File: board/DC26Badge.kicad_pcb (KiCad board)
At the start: 2 copper layers, 6 parts, among them U1 HT16K33-28

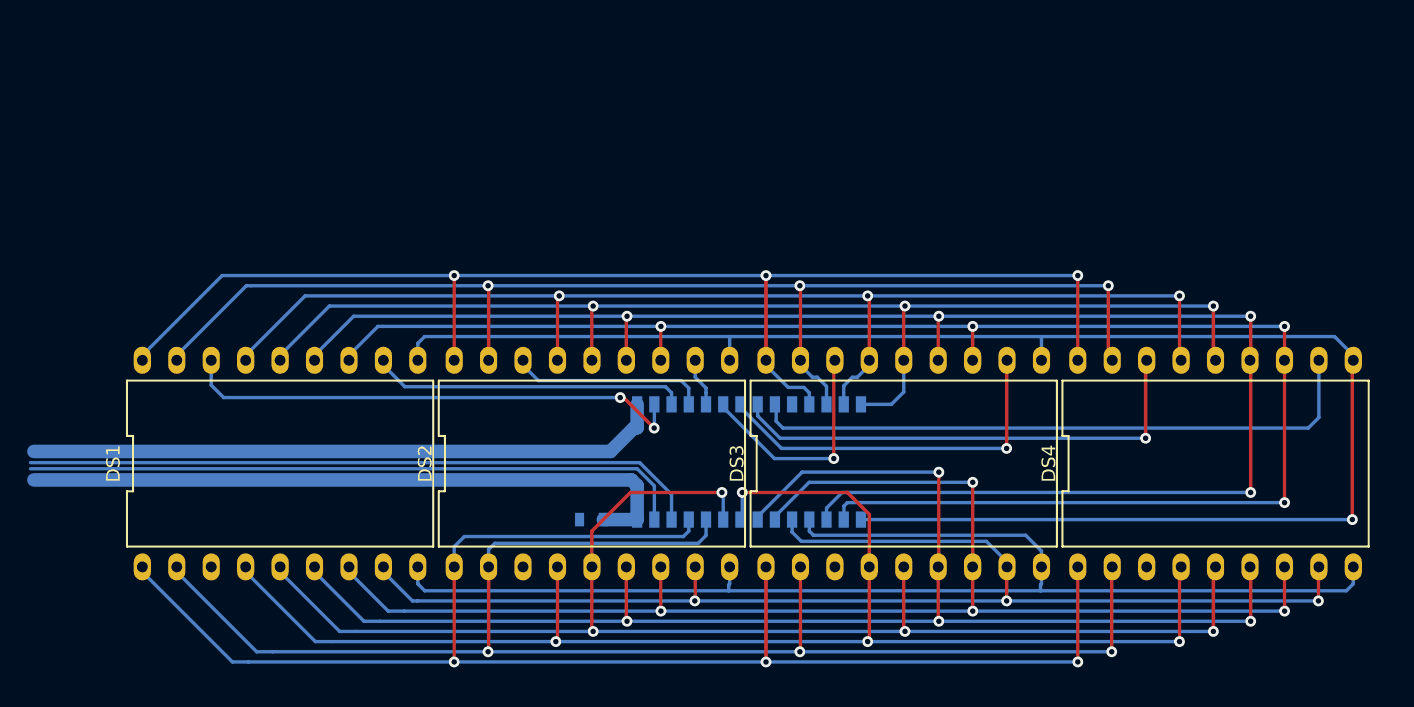
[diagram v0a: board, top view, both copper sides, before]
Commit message: First pass of prototype PCB layout.
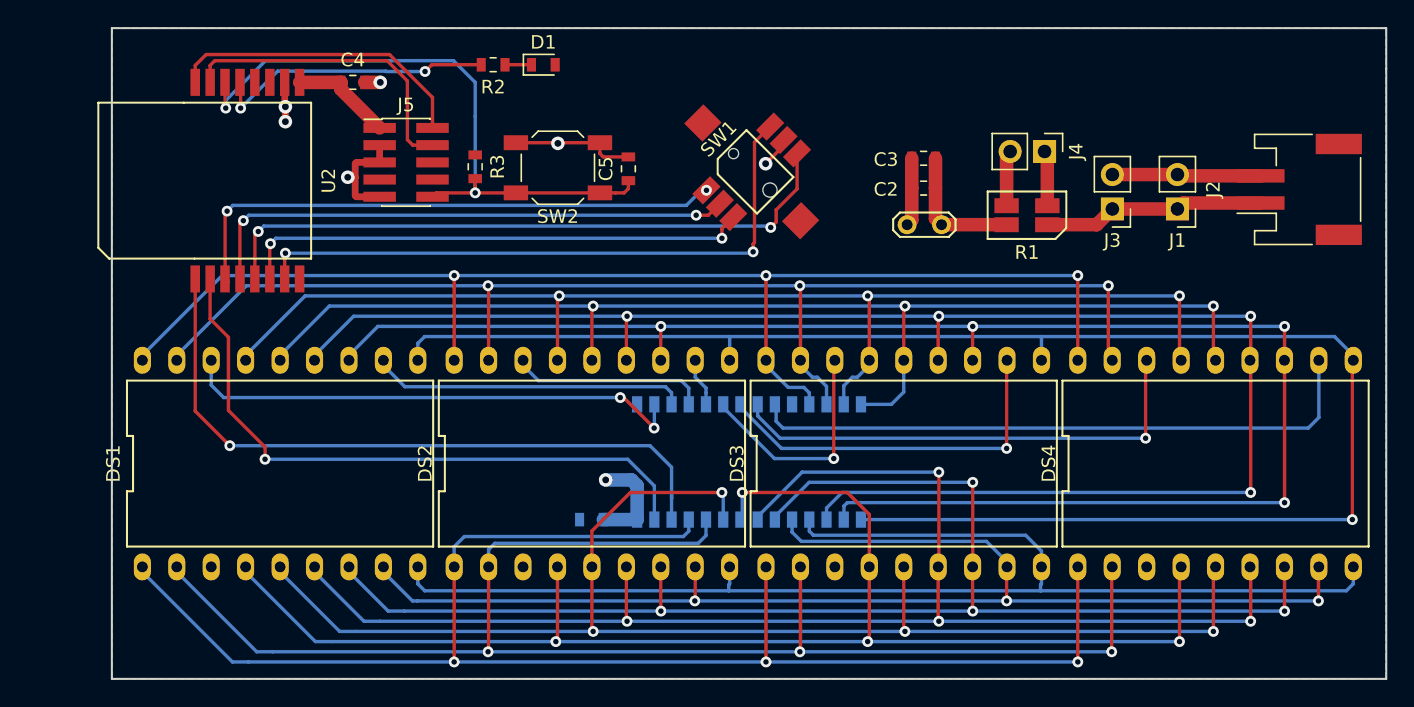
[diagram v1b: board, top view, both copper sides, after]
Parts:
- added C2: 4.7u, Capacitor_SMD:C_0603_1608Metric, F.Cu at (154.9, 33.8)
- added C3: 0.1u, Capacitor_SMD:C_0603_1608Metric, F.Cu at (154.9, 31.6)
- added C4: 0.1u, Capacitor_SMD:C_0603_1608Metric, F.Cu at (112.8, 26.0)
- added C5: 0.1u, Capacitor_SMD:C_0603_1608Metric, F.Cu at (133.1, 32.4)
- added D1: LED, LED_SMD:LED_0603_1608Metric, F.Cu at (126.8, 24.7)
- added J1: PWR_HDR, PinHeaders:Pin_Header_Straight_1x02_Pitch2.54mm, F.Cu at (173.6, 35.3)
- added J2: PWR_CONN, Connector_JST:JST_PH_S2B-PH-SM4-TB_1x02_P2.00mm_Horizontal, F.Cu at (182.6, 33.9)
- added J3: VOLTMETER, PinHeaders:Pin_Header_Straight_1x02_Pitch2.54mm, F.Cu at (168.8, 35.3)
- added J4: AMMETER, PinHeaders:Pin_Header_Straight_1x02_Pitch2.54mm, F.Cu at (163.8, 31.1)
- added J5: Cortex_SWD, Connector_PinHeader_1.27mm:PinHeader_2x05_P1.27mm_Vertical_SMD, F.Cu at (116.7, 31.9)
- added R1: 0.1, DC26badge:FC4T, F.Cu at (162.5, 35.8)
- added R2: 1k, Resistor_SMD:R_0603_1608Metric, F.Cu at (123.1, 24.7)
- added R3: 1k, Resistor_SMD:R_0603_1608Metric, F.Cu at (121.8, 32.2)
- added SW1: JOYSTICK, DC26badge:JOYSTICK, F.Cu at (142.2, 32.6)
- added SW2: SW_Push, Button_Switch_SMD:SW_SPST_SKQG, F.Cu at (127.9, 32.3)
- added TP1: PWRTP, TestPoint:TestPoint_2Pads_Pitch2.54mm_Drill0.8mm, F.Cu at (153.7, 36.5)
- added U2: BT832, DC26badge:BT832, F.Cu at (105.0, 33.2)
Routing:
- net /DN: track 0.00 -> 47.9 mm, vias 0 -> 2
- net /RESET: track 0.00 -> 47.3 mm, vias 0 -> 2
- net /RT: track 0.00 -> 46.2 mm, vias 0 -> 2
- net /UP: track 0.00 -> 41.7 mm, vias 0 -> 2
- net /CTR: track 0.00 -> 40.1 mm, vias 0 -> 2
- net /LT: track 0.00 -> 38.0 mm, vias 0 -> 2
- net VDD: track 49.7 -> 25.0 mm, vias 0 -> 1
- net /SWDCLK: track 0.00 -> 22.9 mm
- net /SWDIO: track 0.00 -> 22.6 mm
- net /LED1: track 0.00 -> 21.0 mm, vias 0 -> 2
- net /P_IN: track 0.00 -> 16.4 mm
- net GND: track 46.9 -> 39.5 mm, vias 0 -> 6
- net Net-(J4-Pad2): track 0.00 -> 4.11 mm
- net Net-(J4-Pad1): track 0.00 -> 4.08 mm
- net Net-(D1-Pad1): track 0.00 -> 1.95 mm
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- added copper zone on B.Cu, net GND
- added copper zone on F.Cu, net VDD
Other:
- board outline added: 94 x 48 mm
